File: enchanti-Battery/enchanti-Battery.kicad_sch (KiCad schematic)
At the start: 7 parts, among them J1 USB4105-GF-A, U3 USBLC6-2P6

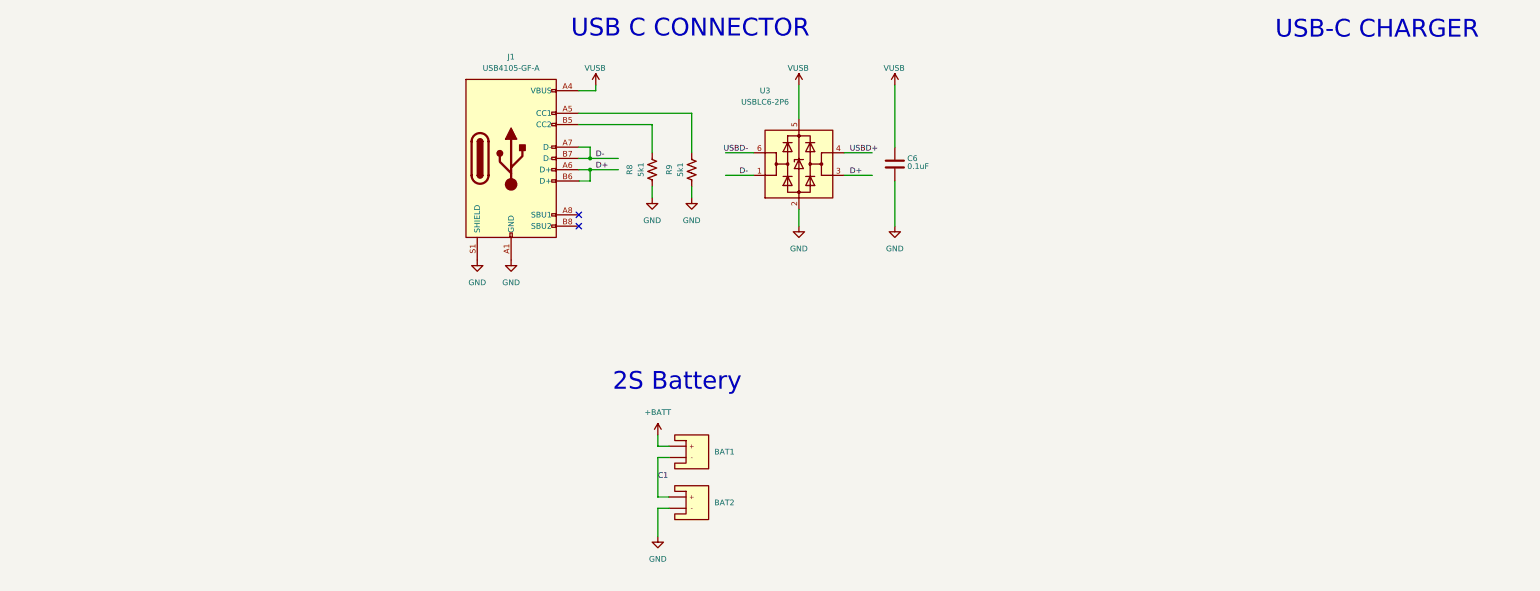
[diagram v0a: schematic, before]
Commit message: Revert "added components to 2S battery charger, changing up the enchanti module design"
This reverts commit 22a1e749752c1cc608d102de7de6baf7b482e290.
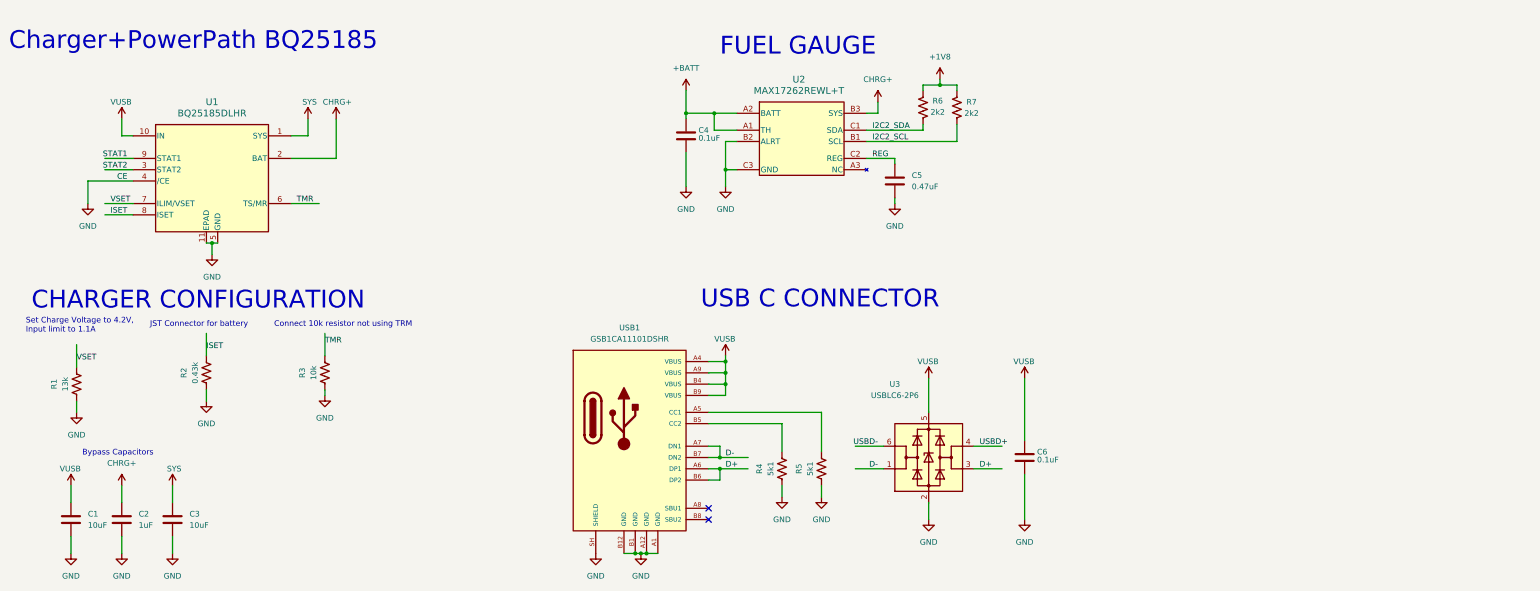
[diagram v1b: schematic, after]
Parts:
- removed BAT1, BAT2: 18650_HOLDER, Battery:BatteryHolder_MPD_BH-18650-PC2, symbol ENCHANTI_connectors:Battery_18650
- removed J1: USB4105-GF-A, Connector_USB:USB_C_Receptacle_GCT_USB4105-xx-A_16P_TopMnt_Horizontal, symbol ENCHANTI_connectors:USB4105-GF-A
- removed R8, R9: 5k1, Resistor_SMD:R_0402_1005Metric, symbol Device:R_US
- added C1, C3: 10uF, Capacitor_SMD:C_0603_1608Metric, symbol Device:C
- added C2: 1uF, Capacitor_SMD:C_0402_1005Metric, symbol Device:C
- added C4: 0.1uF, Capacitor_SMD:C_0402_1005Metric, symbol Device:C
- added C5: 0.47uF, Capacitor_SMD:C_0402_1005Metric, symbol Device:C
- added R1: 13k, Resistor_SMD:R_0402_1005Metric, symbol Device:R_US
- added R2: 0.43k, Resistor_SMD:R_0402_1005Metric, symbol Device:R_US
- added R3: 10k, Resistor_SMD:R_0402_1005Metric, symbol Device:R_US
- added R4, R5: 5k1, Resistor_SMD:R_0402_1005Metric, symbol Device:R_US
- added R6, R7: 2k2, Resistor_SMD:R_0402_1005Metric, symbol Device:R_US
- added SYS1, SYS2: SYS, symbol power-symbols:VSYS
- added U1: BQ25185DLHR, ENCHANTI_battery-management:WSON10_DLH_TEX, symbol ENCHANTI_battery-management:BQ25185DLHR
- added U2: MAX17262REWL+T, ENCHANTI_battery-management:MAX17262, symbol ENCHANTI_battery-management:MAX17262REWL+T
- added USB1: GSB1CA11101DSHR, ENCHANTI_connectors:AMPHENOL_GSB1CA11101DSHR, symbol ENCHANTI_connectors:GSB1CA11101DSHR
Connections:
- net +BATT: now also C4.1, U2.A1 (TH), U2.A2 (BATT)
- net D+: now also USB1.A6 (DP1), USB1.B6 (DP2)
- net D-: now also USB1.A7 (DN1), USB1.B7 (DN2)
- net GND: now also C1.2, C2.2, C3.2, C4.2, C5.2, R1.1, R2.1, R3.1, R4.1, R5.1, U1.11 (EPAD), U1.4 (/CE), U1.5 (GND), U2.B2 (ALRT), U2.C3 (GND), USB1.A1 (GND), USB1.A12 (GND), USB1.B1 (GND), USB1.B12 (GND), USB1.SH (SHIELD)
- net VUSB: now also C1.1, U1.10 (IN), USB1.A4 (VBUS), USB1.A9 (VBUS), USB1.B4 (VBUS), USB1.B9 (VBUS)
- new net: R5.2, USB1.A5 (CC1)
- new net: R4.2, USB1.B5 (CC2)
- new net +1V8: R6.2, R7.2
- new net CHRG+: C2.1, U1.2 (BAT), U2.B3 (SYS)
- new net I2C2_SCL: R7.1, U2.B1 (SCL)
- new net I2C2_SDA: R6.1, U2.C1 (SDA)
- new net ISET: R2.2, U1.8 (ISET)
- new net REG: C5.1, U2.C2 (REG)
- new net STAT1: U1.9 (STAT1)
- new net STAT2: U1.3 (STAT2)
- new net SYS: C3.1, SYS1.1 (SYS), SYS2.1 (SYS), U1.1 (SYS)
- new net TMR: R3.2, U1.6 (TS/MR)
- new net VSET: R1.2, U1.7 (ILIM/VSET)
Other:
- note added: "Bypass Capacitors"
- note added: "CHARGER CONFIGURATION"
- note added: "Charger+PowerPath BQ25185"
- note added: "Connect 10k resistor not using TRM"
- note added: "FUEL GAUGE"
- note added: "JST Connector for battery"
- note added: "Set Charge Voltage to 4.2V, Input limit to 1.1A"
- note removed: "2S Battery"
- note removed: "USB-C CHARGER"
- moved on the sheet: C6, U3
